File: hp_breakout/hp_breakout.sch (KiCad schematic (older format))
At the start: 20 parts, among them J1 AudioJack2_Ground_Switch, J10 Conn_01x05_Male, J11 AudioJack2_Ground_Switch, J12 AudioJack2_Ground_Switch, J13 AudioJack2_Ground_Switch, J14 AudioJack2_Ground_Switch, J15 AudioJack2_Ground_Switch, J16 Conn_01x05_Male, J17 Conn_01x05_Male, J18 Conn_01x05_Male, J19 Conn_01x05_Male, J2 Conn_01x05_Male, J20 Conn_01x05_Male, J3 AudioJack2_Ground_Switch, J4 AudioJack2_Ground_Switch, J5 AudioJack2_Ground_Switch, J6 AudioJack2_Ground_Switch, J7 Conn_01x05_Male, J8 Conn_01x05_Male, J9 Conn_01x05_Male

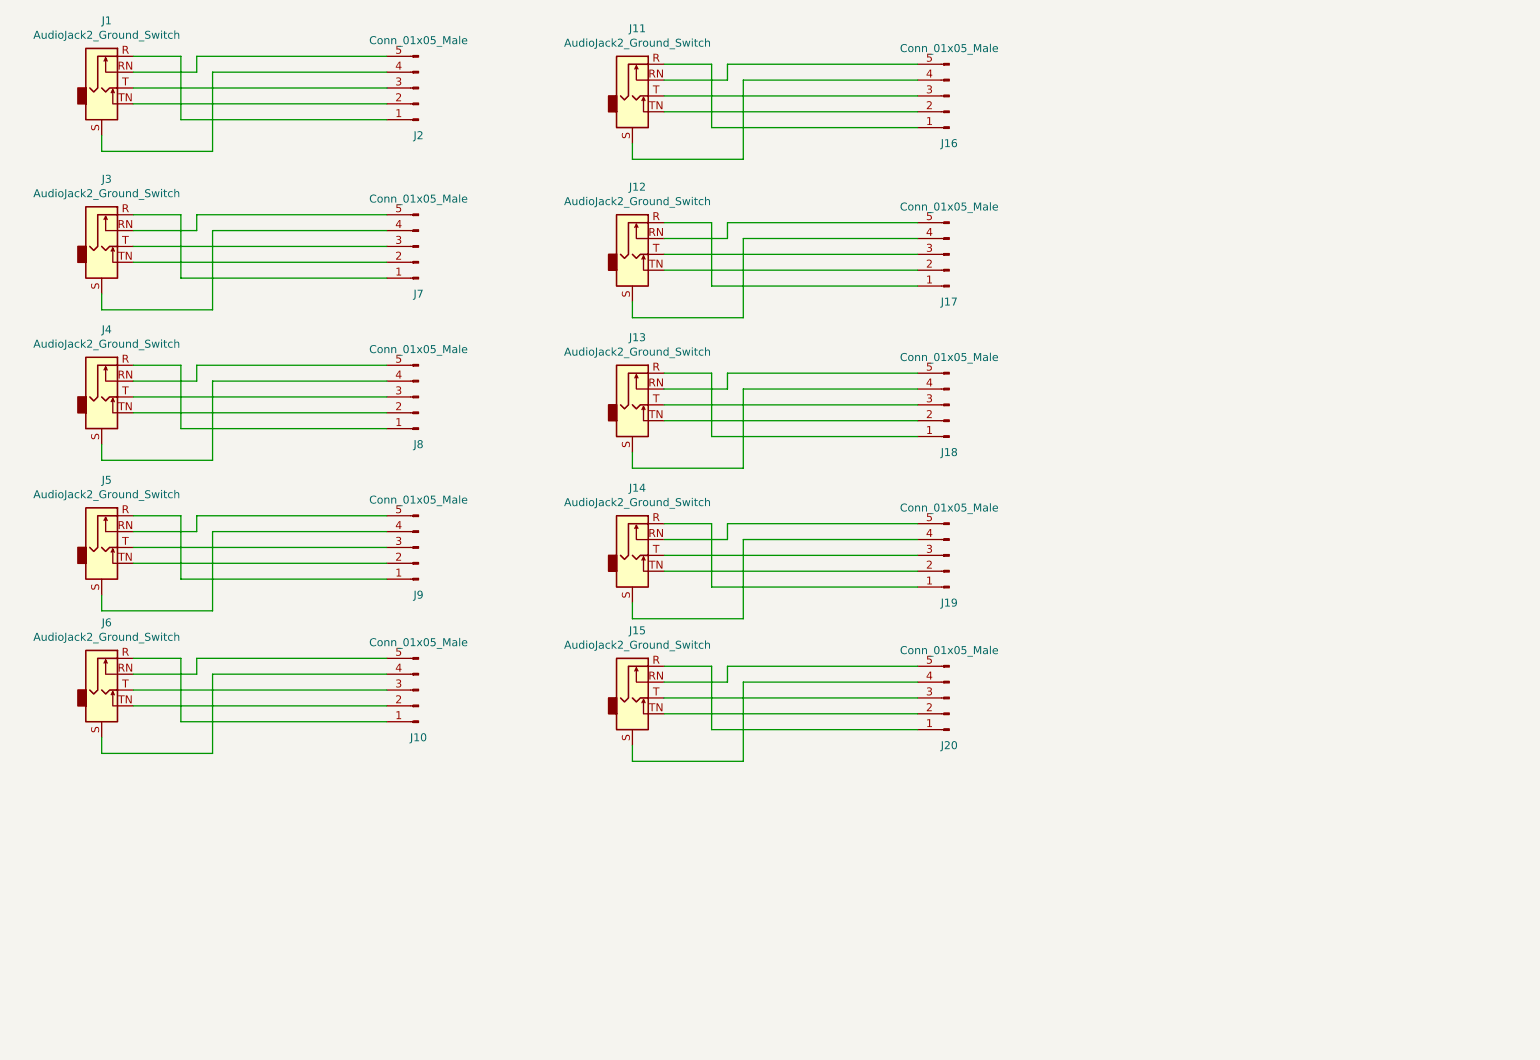
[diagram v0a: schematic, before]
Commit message: 10 identical boards
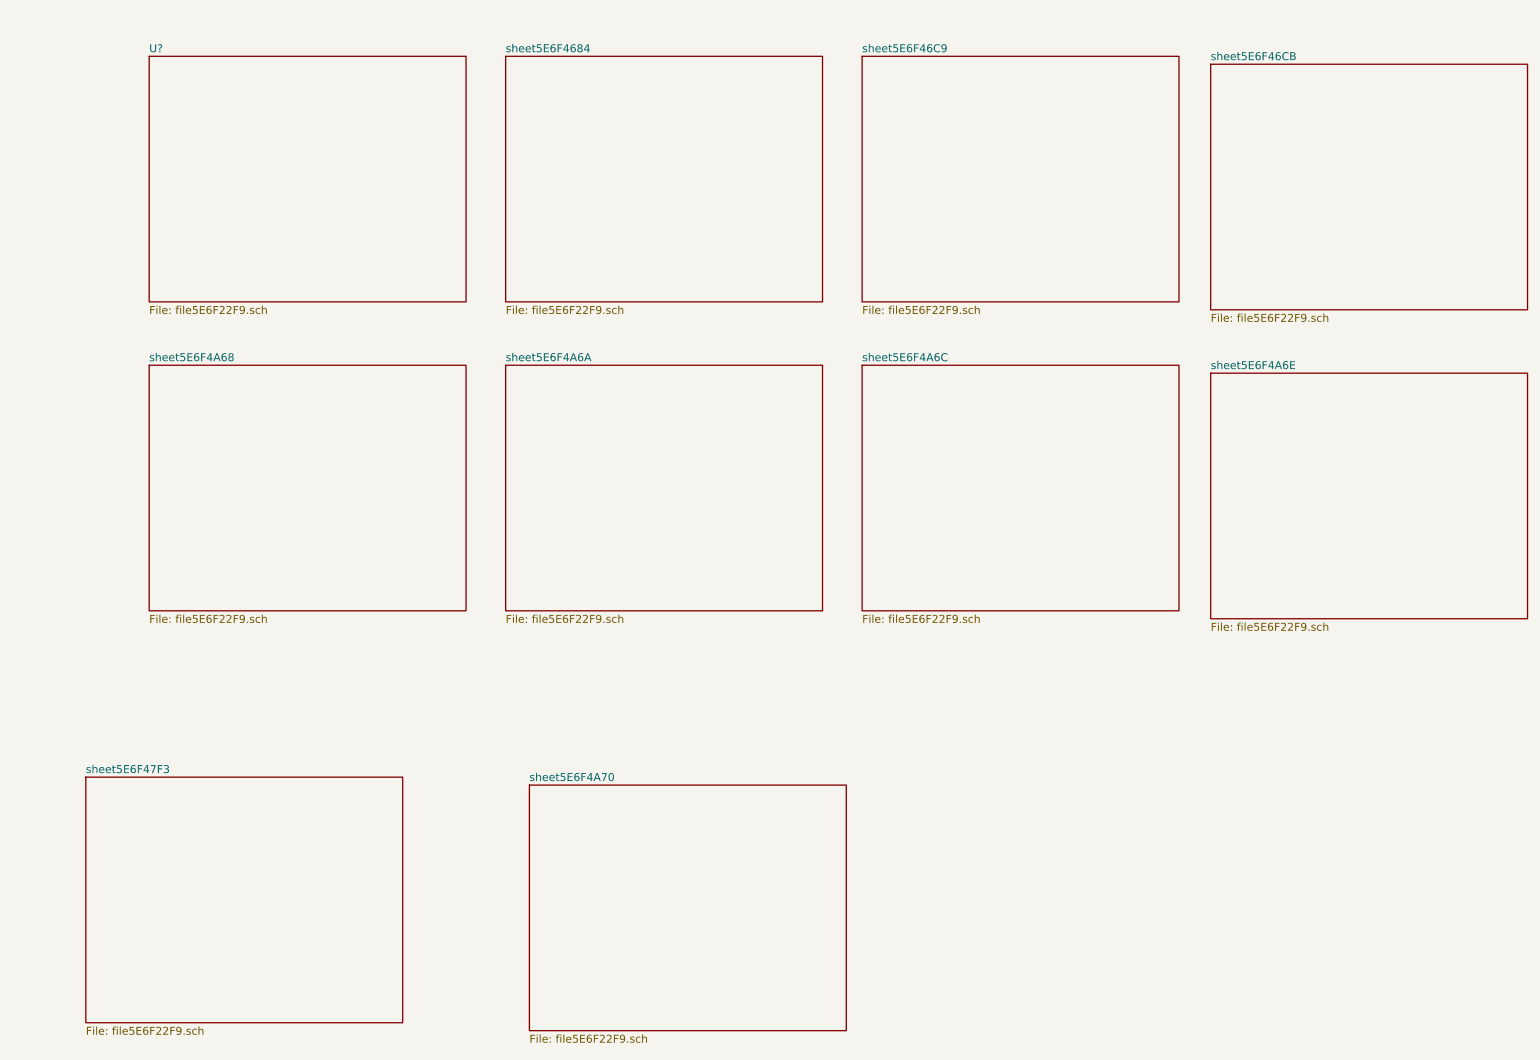
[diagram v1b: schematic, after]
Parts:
- removed J1, J11, J12, J13, J14, J15, J3, J4, J5, J6: AudioJack2_Ground_Switch, KiCad/kicad-footprints/Connector_Audio.pretty:Jack_3.5mm_Ledino_KB3SPRS_Horizontal, symbol hp_breakout:AudioJack2_Ground_Switch
- removed J10, J16, J17, J18, J19, J2, J20, J7, J8, J9: Conn_01x05_Male, KiCad/kicad-footprints/Connector_PinHeader_2.54mm.pretty:PinHeader_1x05_P2.54mm_Vertical, symbol hp_breakout-rescue:Conn_01x05_Male
